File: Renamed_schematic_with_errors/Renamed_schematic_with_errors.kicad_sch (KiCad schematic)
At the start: 23 parts, among them J1 STEP/DIR, J2 VCC_IO, J3 MISC, P9 VM

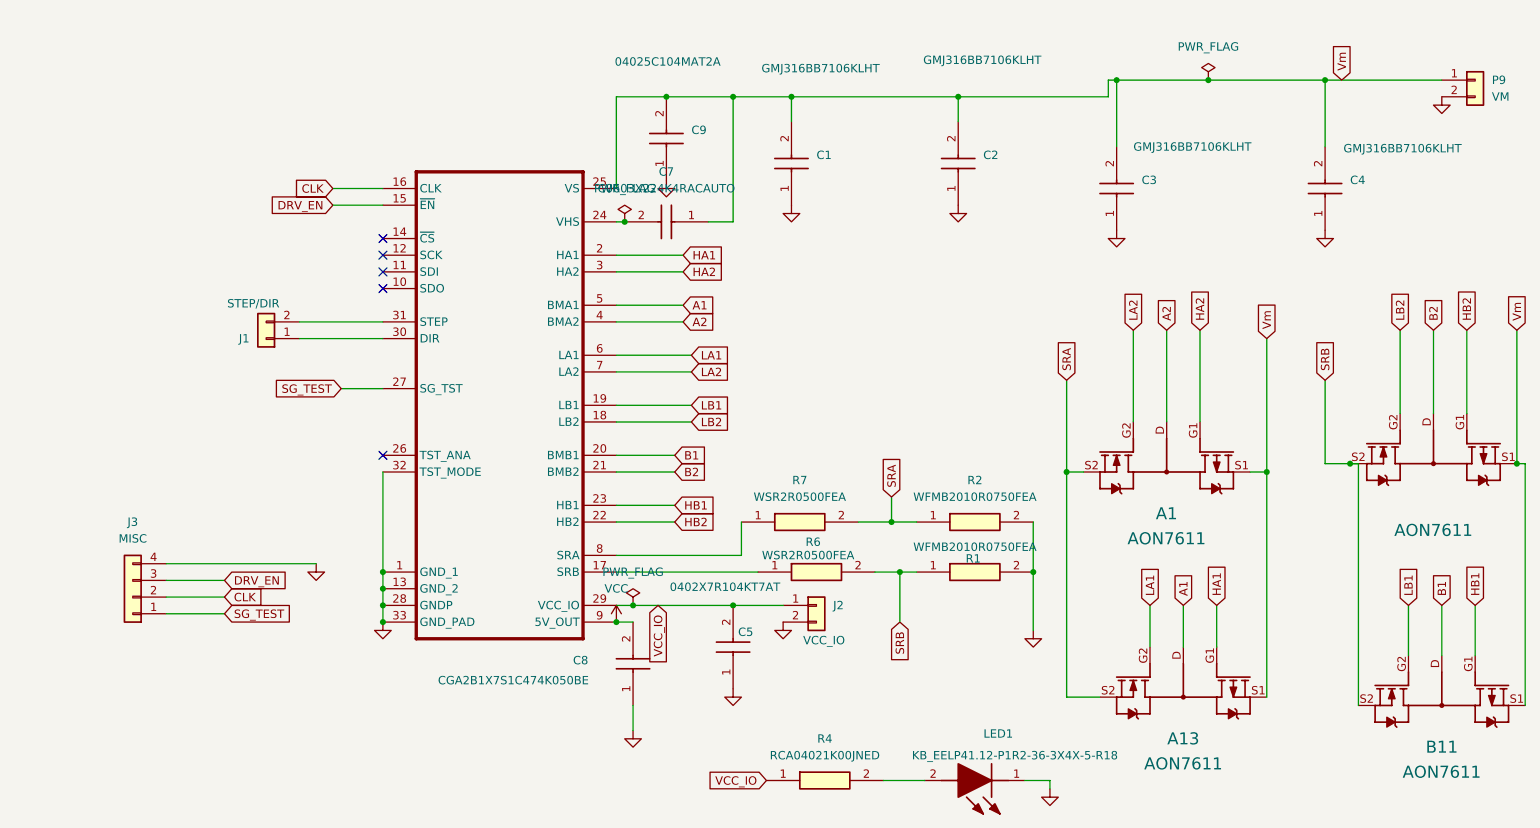
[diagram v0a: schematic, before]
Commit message: this is alot
good luck
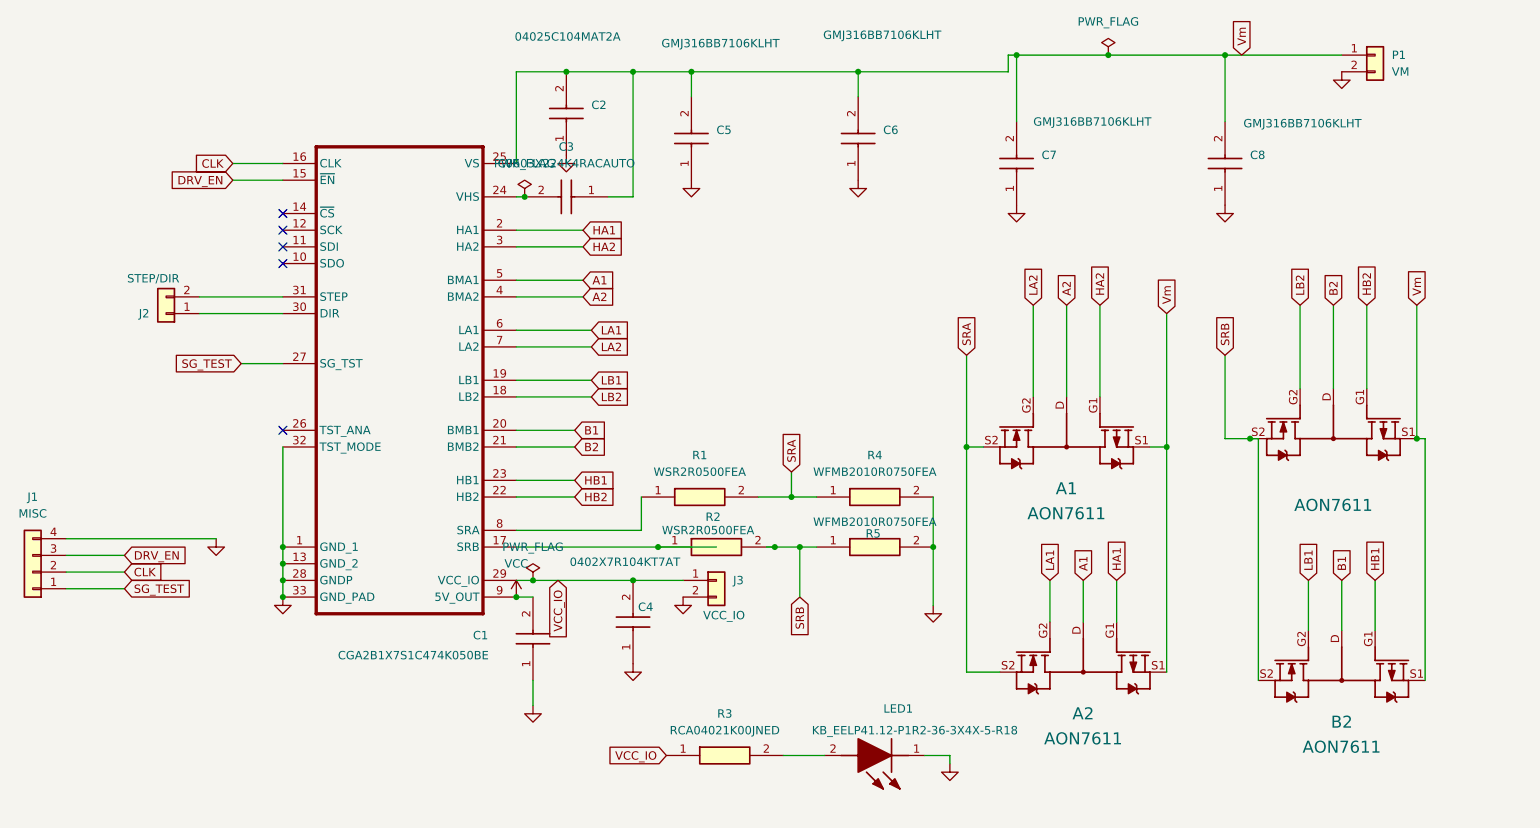
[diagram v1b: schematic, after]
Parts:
- removed A13, B11: AON7611, AON7611, symbol TMC262_BOB40_V1_2:AON7611
- removed C1, C2, C3, C4: GMJ316BB7106KLHT, CAPPC3216X125N, symbol GMJ316BB7106KLHT:GMJ316BB7106KLHT
- removed C5: 0402X7R104KT7AT, CAPC1005X61N, symbol 0402X7R104KT7AT:0402X7R104KT7AT
- removed C7: C0603X224K4RACAUTO, C0603, symbol C0603X224K4RACAUTO:C0603X224K4RACAUTO
- removed C8: CGA2B1X7S1C474K050BE, CAPC1005X55N, symbol CGA2B1X7S1C474K050BE:CGA2B1X7S1C474K050BE
- removed C9: 04025C104MAT2A, CAPC1005X56N, symbol 04025C104MAT2A:04025C104MAT2A
- removed J1: STEP/DIR, symbol Connector_Generic:Conn_01x02
- removed J3: MISC, symbol Connector_Generic:Conn_01x04
- removed P9: VM, symbol Connector_Generic:Conn_01x02
- removed R1, R2: WFMB2010R0750FEA, RESC5125X65N, symbol WFMB2010R0750FEA:WFMB2010R0750FEA
- removed R4: RCA04021K00JNED, RESC1005X40N, symbol RCA04021K00JNED:RCA04021K00JNED
- removed R6, R7: WSR2R0500FEA, RESM11670X254N, symbol WSR2R0500FEA:WSR2R0500FEA
- added A2, B2: AON7611, AON7611, symbol TMC262_BOB40_V1_2:AON7611
- added C1: CGA2B1X7S1C474K050BE, CAPC1005X55N, symbol CGA2B1X7S1C474K050BE:CGA2B1X7S1C474K050BE
- added C2: 04025C104MAT2A, CAPC1005X56N, symbol 04025C104MAT2A:04025C104MAT2A
- added C3: C0603X224K4RACAUTO, C0603, symbol C0603X224K4RACAUTO:C0603X224K4RACAUTO
- added C4: 0402X7R104KT7AT, CAPC1005X61N, symbol 0402X7R104KT7AT:0402X7R104KT7AT
- added C5, C6, C7, C8: GMJ316BB7106KLHT, CAPPC3216X125N, symbol GMJ316BB7106KLHT:GMJ316BB7106KLHT
- added J1: MISC, symbol Connector_Generic:Conn_01x04
- added J3: VCC_IO, symbol Connector_Generic:Conn_01x02
- added P1: VM, symbol Connector_Generic:Conn_01x02
- added R1, R2: WSR2R0500FEA, RESM11670X254N, symbol WSR2R0500FEA:WSR2R0500FEA
- added R3: RCA04021K00JNED, RESC1005X40N, symbol RCA04021K00JNED:RCA04021K00JNED
- added R4, R5: WFMB2010R0750FEA, RESC5125X65N, symbol WFMB2010R0750FEA:WFMB2010R0750FEA
- J2: value VCC_IO -> STEP/DIR
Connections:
- net A1: now also A2.D
- net B1: now also B2.D
- net CLK: now also J1.2 (Pin_2)
- net DRV_EN: now also J1.3 (Pin_3)
- net GND: now also C1.1, C2.1, C4.1, C5.1, C6.1, C7.1, C8.1, J1.4 (Pin_4), J3.2 (Pin_2), P1.2 (Pin_2), R4.2, R5.2; no longer J2.2 (Pin_2)
- net HA1: now also A2.G1
- net HB1: now also B2.G1
- net LA1: now also A2.G2
- net LB1: now also B2.G2
- net SG_TEST: now also J1.1 (Pin_1)
- net SRA: now also A2.S2, R1.2, R4.1
- net SRB: now also B2.S2, R2.2, R5.1
- net VCC: now also C1.2
- net VCC_IO: now also C4.2, J3.1 (Pin_1), R3.1; no longer J2.1 (Pin_1)
- net Vm: now also A2.S1, B2.S1, C2.2, C3.1, C5.2, C6.2, C7.2, C8.2, P1.1 (Pin_1)
- net at IC1.24 (VHS): now also C3.2
- net at IC1.8 (SRA): now also R1.1
- net at IC1.17 (SRB): now also R2.1
- net at IC1.30 (DIR): now also J2.1 (Pin_1)
- net at IC1.31 (STEP): now also J2.2 (Pin_2)
- net at LED1.2 (A): now also R3.2
